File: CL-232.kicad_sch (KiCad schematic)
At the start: 42 parts, among them J1 Conn_01x06, J2 Screw_Terminal_01x10, J3 Barrel_Jack_Switch, J4 DE9_Socket_MountingHoles, J5 DB25_Socket, J6 Conn_01x03, J7 Conn_01x01, Q1 2N3904, Q2 2N3904, Q3 2N3904, Q4 2N3906, Q5 2N3904, U1 6N135, U2 4N35, U3 LM7805_TO220, U4 MAX3232

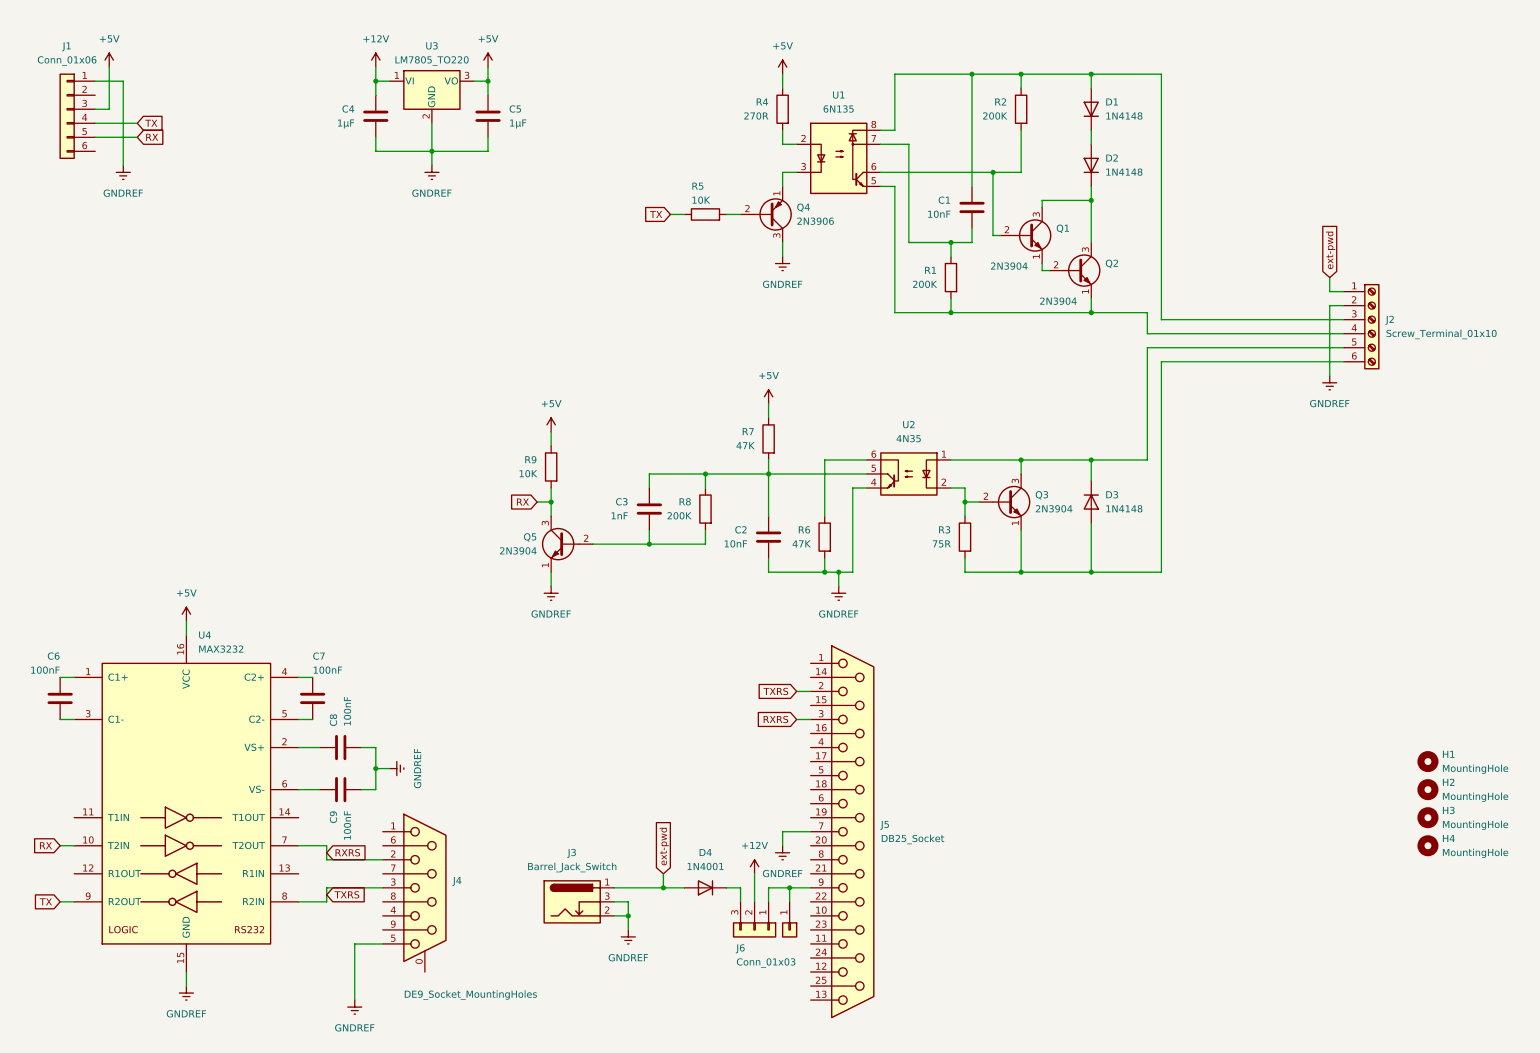
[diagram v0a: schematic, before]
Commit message: First Draft
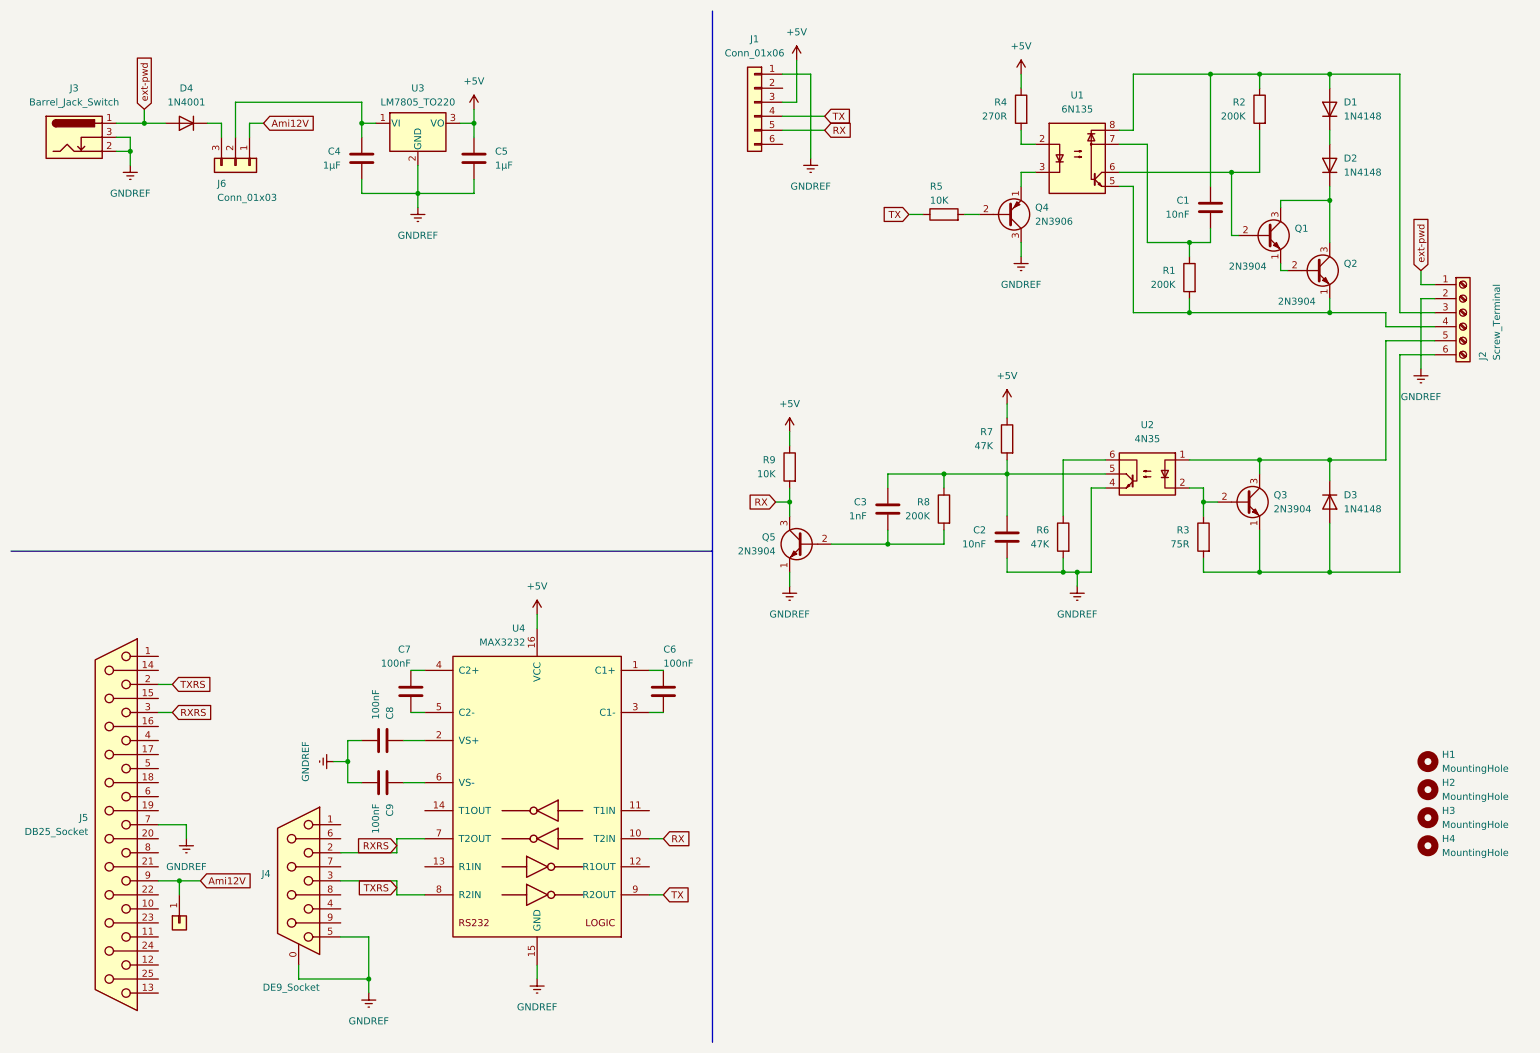
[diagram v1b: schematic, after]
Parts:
- J2: value Screw_Terminal_01x10 -> Screw_Terminal
- J4: value DE9_Socket_MountingHoles -> DE9_Socket
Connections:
- net GNDREF: now also J4.0 (PAD)
- net Ami12V: now reaches J5.9, J6.1 (Pin_1), J7.1 (Pin_1)
- net +12V: no longer names the net of C4.1, J6.2 (Pin_2), U3.1 (VI)
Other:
- moved on the sheet: C1, C2, C3, C4, C5, C6, C7, C8, C9, D1, D2, D3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
